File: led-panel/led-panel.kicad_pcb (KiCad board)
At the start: 2 copper layers, 83.8 x 50.8 mm, 129 parts, among them J1 Conn_01x24

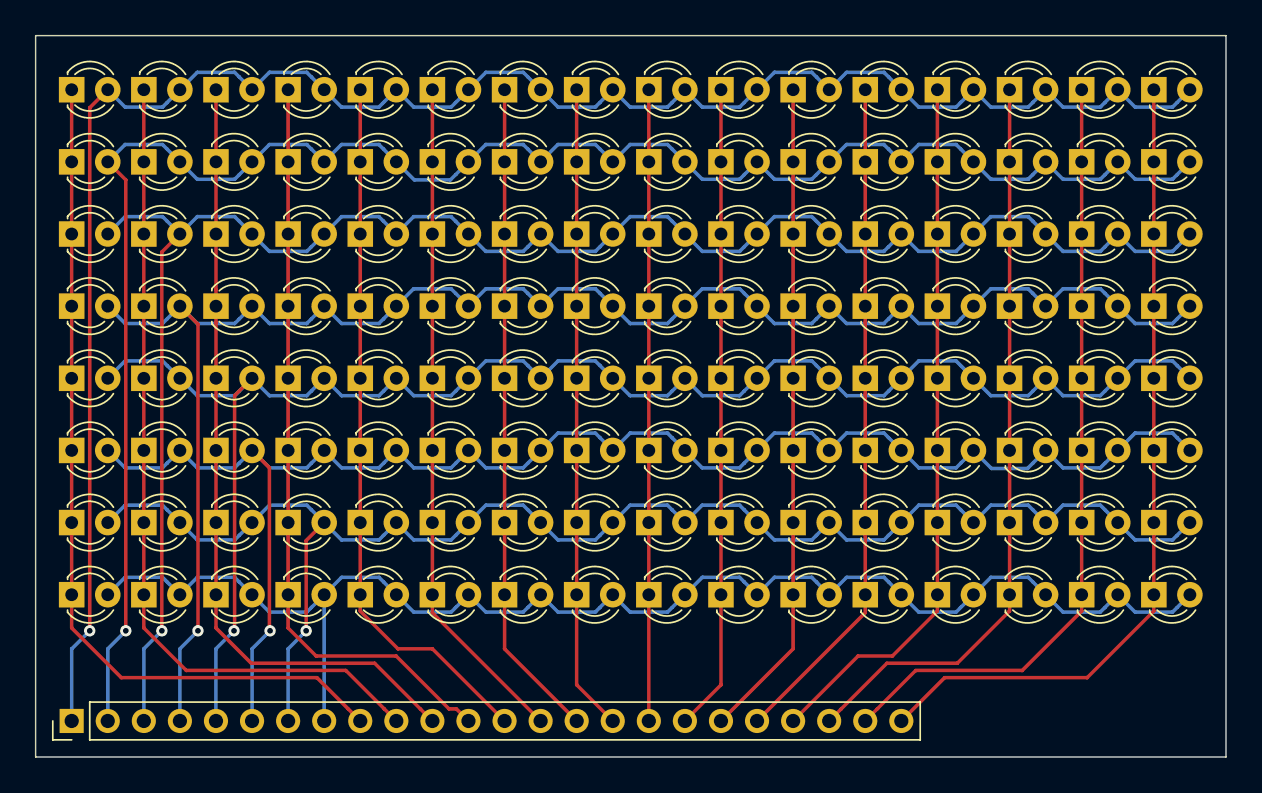
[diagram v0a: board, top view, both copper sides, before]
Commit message: fix the routing
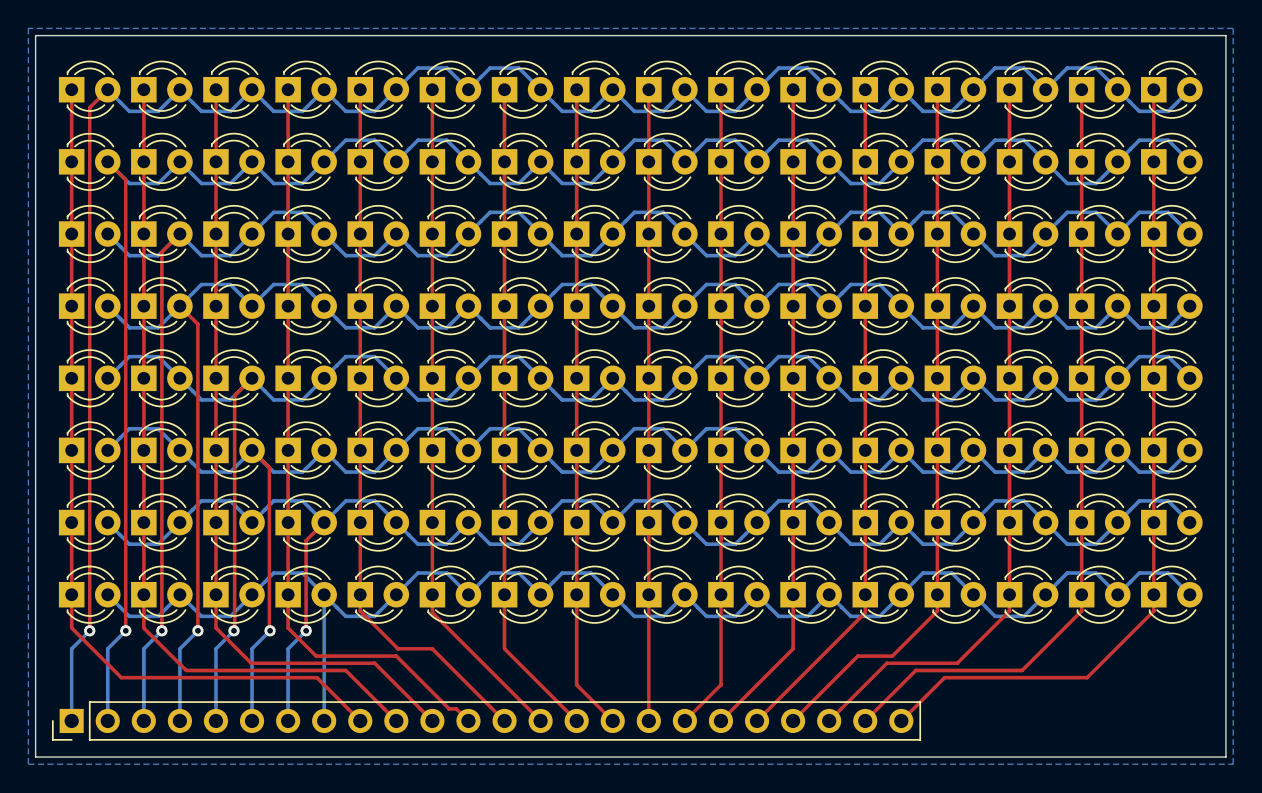
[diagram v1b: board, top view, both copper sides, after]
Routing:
- net Net-(D10-Pad2): track 126.8 -> 130.5 mm
- net Net-(D103-Pad2): track 100.3 -> 104.0 mm
- net Net-(D102-Pad2): track 106.4 -> 110.2 mm
- net Net-(D107-Pad2): track 121.7 -> 125.4 mm
- net Net-(D0-Pad2): track 136.9 -> 140.6 mm
- net Net-(D100-Pad2): track 116.6 -> 120.3 mm
- net Net-(D101-Pad2): track 111.6 -> 115.2 mm
- net Net-(D1-Pad2): track 131.9 -> 135.6 mm
- added copper zone on B.Cu, net (none)
